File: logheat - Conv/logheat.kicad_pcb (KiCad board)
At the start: 2 copper layers, 85 x 55 mm, 27 parts, among them J1 Conn_01x05_MountingPin, J2 Conn_01x02, J3 Conn_01x04_MountingPin, J4 Conn_01x04_MountingPin, J5 Conn_01x04_MountingPin, J6 Conn_01x02, J7 Conn_01x04_MountingPin, J8 Conn_01x04_MountingPin, J9 Conn_01x04_MountingPin, U1 AD8603AUJZ-R2, U2 MCP3004-I_P, U3 AD8603AUJZ-R2, U4 AD8603AUJZ-R2

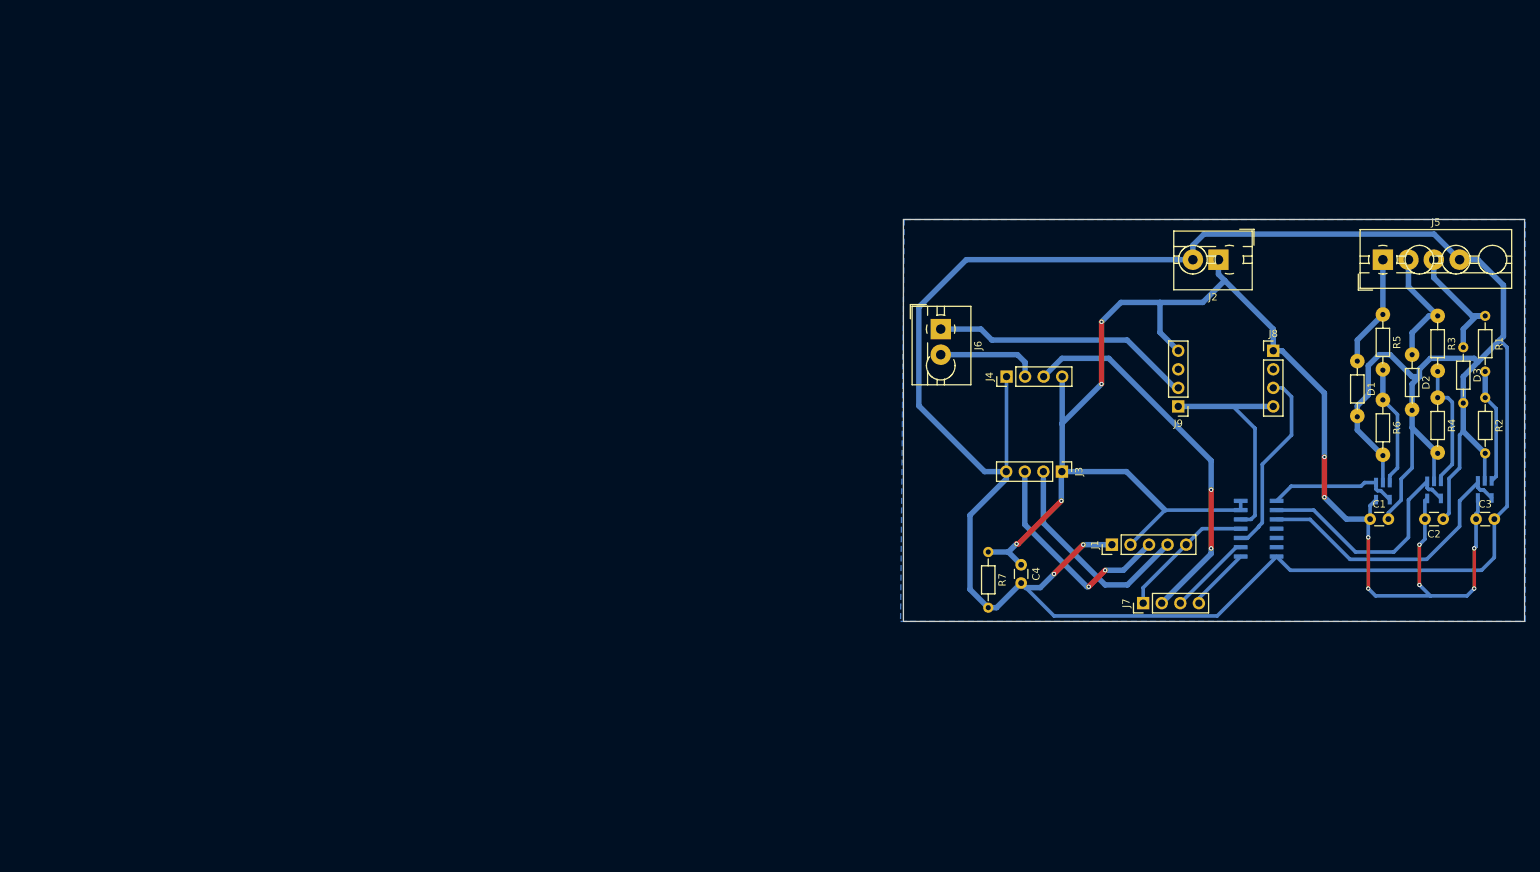
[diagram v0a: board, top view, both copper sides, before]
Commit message: mcp_board
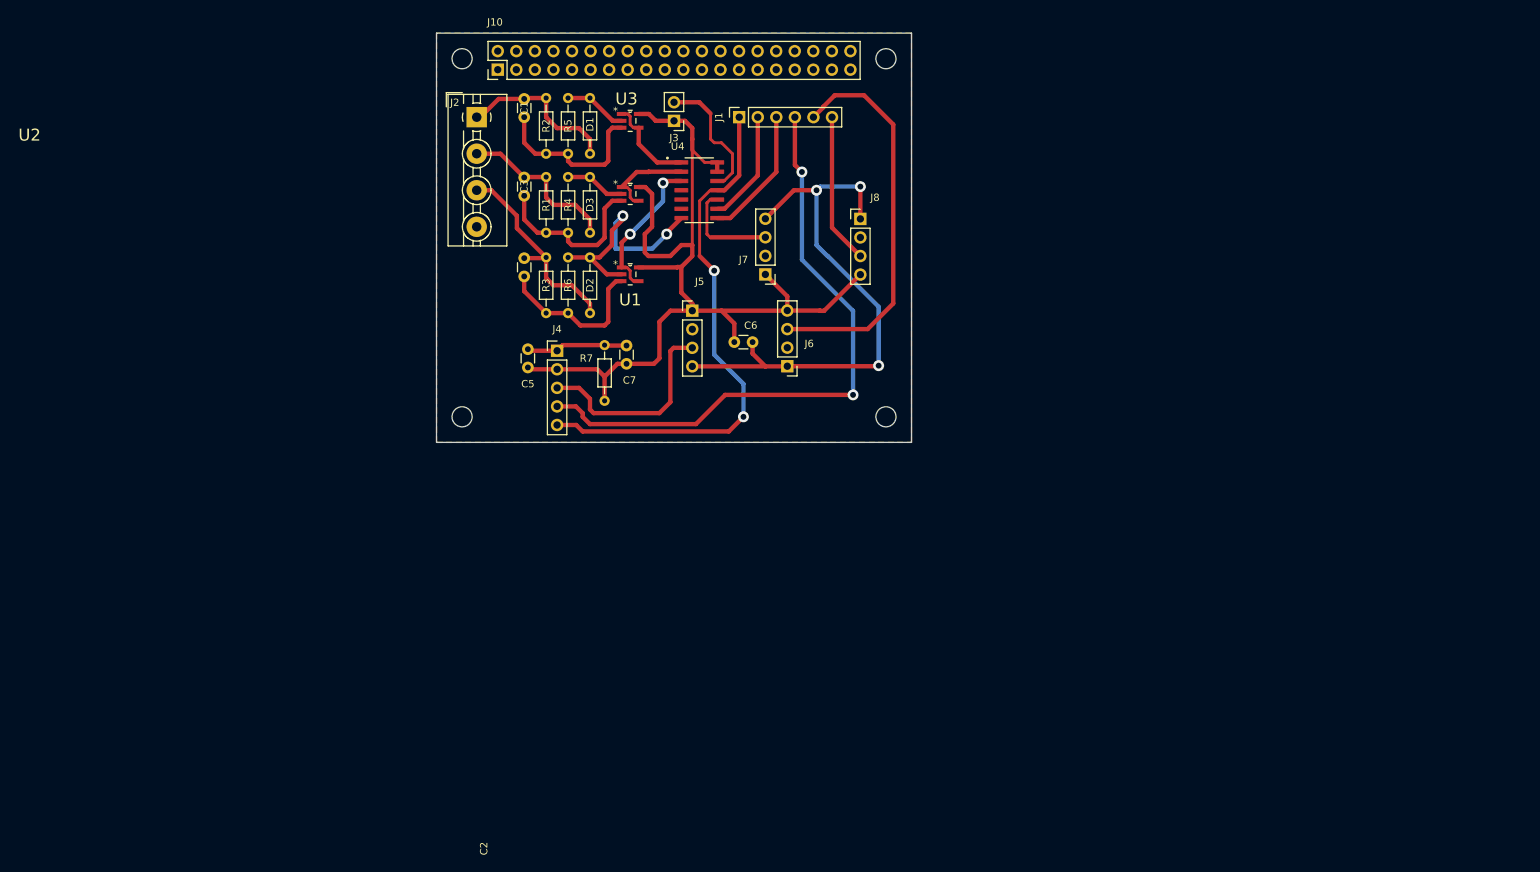
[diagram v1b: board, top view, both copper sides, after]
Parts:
- removed C4: C, Capacitor_THT:C_Disc_D3.0mm_W1.6mm_P2.50mm
- removed J9: Conn_01x04_MountingPin, Connector_PinHeader_2.54mm:PinHeader_1x04_P2.54mm_Vertical
- added ?: , , F.Cu at (23.5, 23.5)
- added ?: , , F.Cu at (81.5, 23.5)
- added ?: , , F.Cu at (23.5, 72.5)
- added ?: , , F.Cu at (81.5, 72.5)
- added C5: C, Capacitor_THT:C_Disc_D3.0mm_W1.6mm_P2.50mm, F.Cu at (32.5, 65.8)
- added C6: C, Capacitor_THT:C_Disc_D3.0mm_W1.6mm_P2.50mm, F.Cu at (60.8, 62.3)
- added C7: C, Capacitor_THT:C_Disc_D3.0mm_W1.6mm_P2.50mm, F.Cu at (46.0, 65.2)
- added J10: Raspberry_Pi_4, Connector_PinHeader_2.54mm:PinHeader_2x20_P2.54mm_Vertical, F.Cu at (28.4, 25.0)
- J1: value Conn_01x05_MountingPin -> Conn_01x06_MountingPin; footprint Connector_PinHeader_2.54mm:PinHeader_1x05_P2.54mm_Vertical -> Connector_PinSocket_2.54mm:PinSocket_1x06_P2.54mm_Vertical
- J2: value Conn_01x02 -> Analog_inputs; footprint TerminalBlock:TerminalBlock_MaiXu_MX126-5.0-02P_1x02_P5.00mm -> TerminalBlock:TerminalBlock_MaiXu_MX126-5.0-04P_1x04_P5.00mm
- J3: value Conn_01x04_MountingPin -> Conn_01x02_MountingPin; footprint Connector_PinHeader_2.54mm:PinHeader_1x04_P2.54mm_Vertical -> Connector_PinHeader_2.54mm:PinHeader_1x02_P2.54mm_Vertical
- J4: value Conn_01x04_MountingPin -> Circuit_conditiono; footprint Connector_PinHeader_2.54mm:PinHeader_1x04_P2.54mm_Vertical -> Connector_PinHeader_2.54mm:PinHeader_1x05_P2.54mm_Vertical
- J5: value Conn_01x04_MountingPin -> protec_condit; footprint TerminalBlock:TerminalBlock_MaiXu_MX126-5.0-04P_1x04_P5.00mm -> Connector_PinHeader_2.54mm:PinHeader_1x04_P2.54mm_Vertical
- J6: value Conn_01x02 -> protec_condit; footprint TerminalBlock:TerminalBlock_MaiXu_MX126-5.0-02P_1x02_P5.00mm -> Connector_PinHeader_2.54mm:PinHeader_1x04_P2.54mm_Vertical
- J7, J8: value Conn_01x04_MountingPin -> protec_mcp
- U1, U3: moved to F.Cu
- U2: value MCP3004-I_P -> AD8603AUJZ-R2; footprint Library:MCP3004 ISL -> Library:AD3603; moved to F.Cu
- U4: value AD8603AUJZ-R2 -> MCP3004-I_P; footprint Library:AD3603 -> Library:MCP3004 ISL; moved to F.Cu
- moved C3 137.6 mm to (32.0, 42.2), turned to 90 degrees
- moved R2 134.9 mm to (35.0, 28.9)
- moved C2 130.1 mm to (32.0, 53.3), turned to 90 degrees
- moved R1 129.9 mm to (35.0, 39.7)
- moved C1 128.2 mm to (32.0, 31.5), turned to 90 degrees
- moved R3 122.3 mm to (35.0, 50.7)
- moved R4 121.1 mm to (38.0, 47.3), turned to 90 degrees
- moved U3 121.0 mm to (46.5, 32.0), turned to 0 degrees
- moved U1 120.6 mm to (46.5, 53.0), turned to 0 degrees
- moved D3 120.5 mm to (41.0, 47.3), turned to 90 degrees
- moved R5 113.6 mm to (38.0, 36.5), turned to 90 degrees
- moved D2 112.6 mm to (41.0, 58.3), turned to 90 degrees
- moved R6 112.1 mm to (38.0, 58.3), turned to 90 degrees
- moved D1 108.8 mm to (41.0, 36.5), turned to 90 degrees
- moved J2 104.8 mm to (25.5, 31.5), turned to -90 degrees
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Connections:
- C1 pad 1: +3V3 -> Net-(U3-+IN)
- C1 pad 2: GND -> Net-(D1-K)
- C2 pad 1: GND -> Net-(U1-+IN)
- C2 pad 2: +3V3 -> Net-(D2-K)
- C3 pad 1: +3V3 -> Net-(U2-+IN)
- C3 pad 2: GND -> Net-(D3-K)
- J1 pad 1: GND -> Net-(J1-Pin_1)
- J1 pad 2: +3V3 -> Net-(J1-Pin_2)
- J2 pad 1: +3V3 -> Net-(D1-K)
- J2 pad 2: GND -> Net-(D3-K)
- J3 pad 2: Net-(J1-Pin_4) -> GND
- J4 pad 2: Net-(J4-Pin_2) -> +3V3
- J4 pad 4: +3V3 -> Net-(J1-Pin_4)
- J5 pad 1: Net-(D1-K) -> +3V3
- J5 pad 2: Net-(D2-K) -> unconnected-(J5-Pin_2-Pad2)
- J5 pad 3: Net-(D3-K) -> Net-(J4-Pin_3)
- J6 pad 1: Net-(J6-Pin_1) -> GND
- J6 pad 2: Net-(J4-Pin_2) -> unconnected-(J6-Pin_2-Pad2)
- J7 pad 1: Net-(J1-Pin_5) -> +3V3
- J7 pad 2: Net-(J4-Pin_3) -> unconnected-(J7-Pin_2-Pad2)
- J7 pad 4: Net-(J7-Pin_4) -> GND
- J8 pad 1: +3V3 -> GND
- J8 pad 3: Net-(J8-Pin_3) -> Net-(J1-Pin_6)
- J8 pad 4: GND -> +3V3
- R1 pad 2: Net-(U1-+IN) -> Net-(U2-+IN)
- R2 pad 1: Net-(U1-+IN) -> Net-(D1-K)
- R2 pad 2: GND -> Net-(U3-+IN)
- R3 pad 2: Net-(U3-+IN) -> Net-(U1-+IN)
- R4 pad 1: Net-(U3-+IN) -> Net-(U2-+IN)
- R5 pad 1: Net-(D1-K) -> Net-(U3-+IN)
- R5 pad 2: Net-(U4-+IN) -> GND
- R6 pad 1: Net-(U4-+IN) -> Net-(U1-+IN)
- R7 pad 1: +3V3 -> GND
- R7 pad 2: GND -> +3V3
- U2 pad 1: Net-(U2-CH0) -> Net-(U2--IN)
- U2 pad 2: Net-(U2-CH1) -> GND
- U2 pad 3: Net-(U1--IN) -> Net-(U2-+IN)
- U2 pad 4: unconnected-(U2-CH3-Pad4) -> Net-(U2--IN)
- U2 pad 5: unconnected-(U2-NC_2-Pad5) -> +3V3
- U3 pad 1: Net-(U2-CH1) -> Net-(U3--IN)
- U3 pad 4: Net-(U2-CH1) -> Net-(U3--IN)
- U4 pad 1: Net-(U2-CH0) -> Net-(U3--IN)
- U4 pad 2: GND -> Net-(U2--IN)
- U4 pad 3: Net-(U4-+IN) -> Net-(U1--IN)
- U4 pad 4: Net-(U2-CH0) -> /NC
- U4 pad 5: +3V3 -> unconnected-(U4-NC_2-Pad5)
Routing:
- net GND: track 416.6 -> 157.7 mm, vias 2 -> 5
- net +3V3: track 211.7 -> 132.8 mm, vias 12 -> 0
- net Net-(J1-Pin_1): track 0.00 -> 73.5 mm, vias 0 -> 2
- net Net-(J1-Pin_4): track 29.8 -> 84.7 mm, vias 0 -> 2
- net Net-(J6-Pin_1): track 35.8 -> 0.00 mm
- net Net-(J1-Pin_5): track 18.8 -> 54.3 mm
- net Net-(U2-CH1): track 33.4 -> 0.00 mm
- net Net-(J8-Pin_3): track 25.8 -> 0.00 mm
- net Net-(U2-+IN): track 0.00 -> 23.6 mm
- net Net-(J4-Pin_3): track 52.1 -> 28.6 mm, vias 2 -> 0
- net Net-(J1-Pin_6): track 0.00 -> 20.6 mm
- net Net-(U1--IN): track 39.8 -> 20.2 mm, vias 0 -> 2
- net Net-(U2-CH0): track 18.0 -> 0.00 mm
- net Net-(U4-+IN): track 16.6 -> 0.00 mm
- net Net-(J1-Pin_2): track 0.00 -> 15.4 mm
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- added copper zone on F.Cu, net GND
- removed copper zone on B.Cu, net GND
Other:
- board size 85 x 55 mm -> 65 x 56 mm
